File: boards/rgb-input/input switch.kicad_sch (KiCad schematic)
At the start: 5 parts

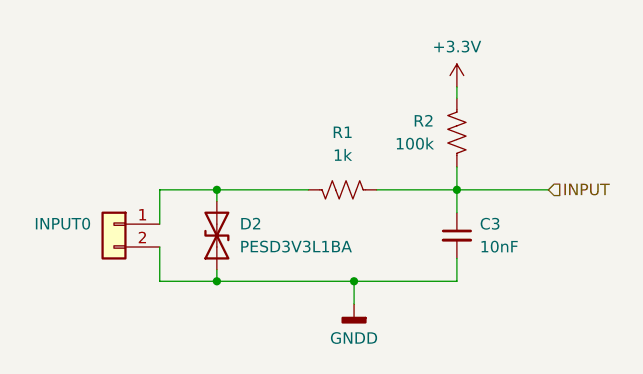
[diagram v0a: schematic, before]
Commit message: passing ERC and DRC
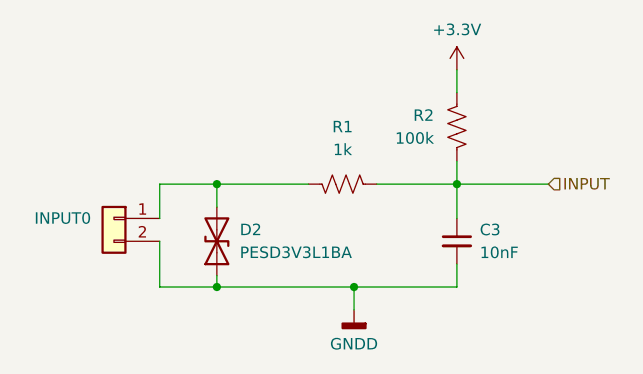
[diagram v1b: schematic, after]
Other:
- moved on the sheet: C3, D2, INPUT0, R1, R2
